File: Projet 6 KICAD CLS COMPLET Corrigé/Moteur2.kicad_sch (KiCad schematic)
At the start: 16 parts

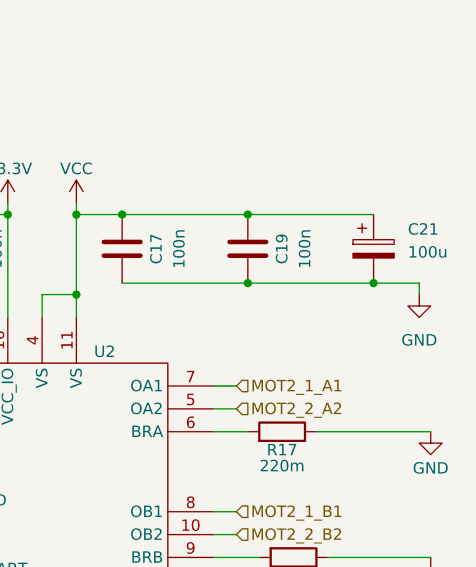
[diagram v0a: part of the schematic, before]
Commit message: Add files via upload
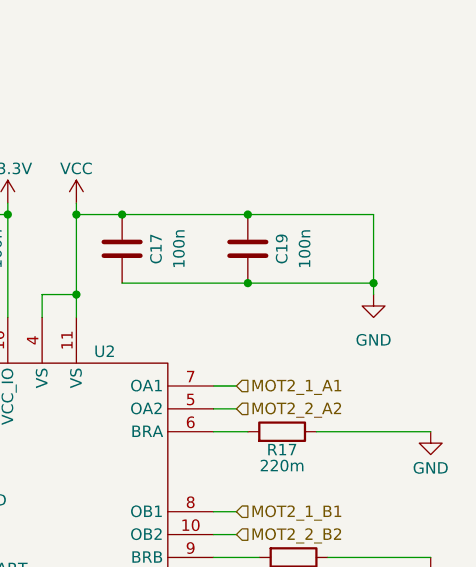
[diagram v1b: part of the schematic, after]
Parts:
- removed C21: 100u, symbol Device:C_Polarized
- C11, C16, C17, C19, C20, C7: footprint (none) -> Capacitor_SMD:C_0805_2012Metric
- D1: footprint (none) -> LED_SMD:LED_0603_1608Metric
- R1, R17, R18, R19, R2, R3, R7: footprint (none) -> Resistor_SMD:R_0603_1608Metric
- U2: footprint (none) -> Package_SO:HTSSOP-28-1EP_4.4x9.7mm_P0.65mm_EP2.85x5.4mm_ThermalVias
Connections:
- net VCC is gone; now on net GND: C11.2, C17.1, C19.1, U2.11 (VS), U2.4 (VS)
